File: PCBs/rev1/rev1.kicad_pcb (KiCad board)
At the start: 2 copper layers, 30.5 x 30.5 mm, 42 parts, among them J1 USB_B_Micro, J2 Conn_01x03, J3 Conn_01x08, J4 Conn_01x05, J5 Conn_01x04, J6 Conn_01x01, SW1 SW_Push, U1 RP2040, U2 AZ1117-3.3, U3 W25Q32JVSS, Y1 12Mhz

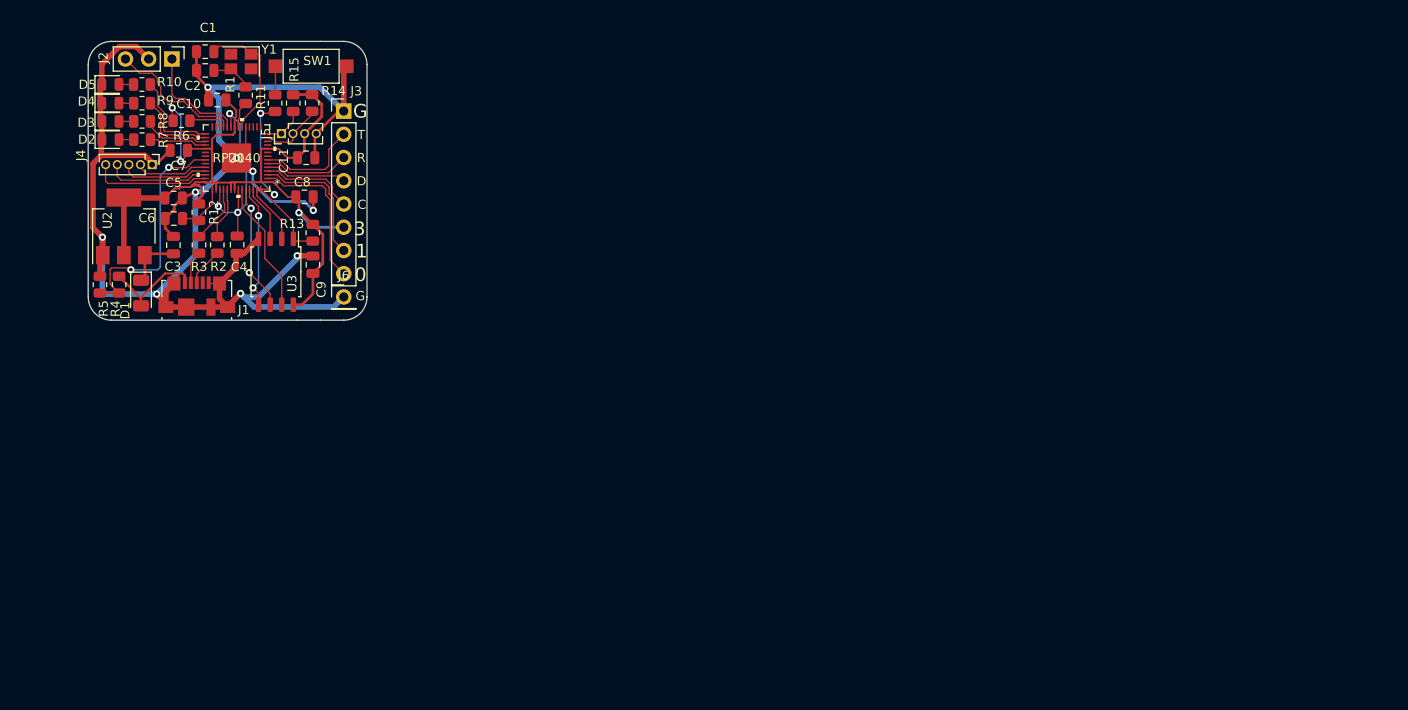
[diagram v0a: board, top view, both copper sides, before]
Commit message: PCB
dhwiqodhiowq
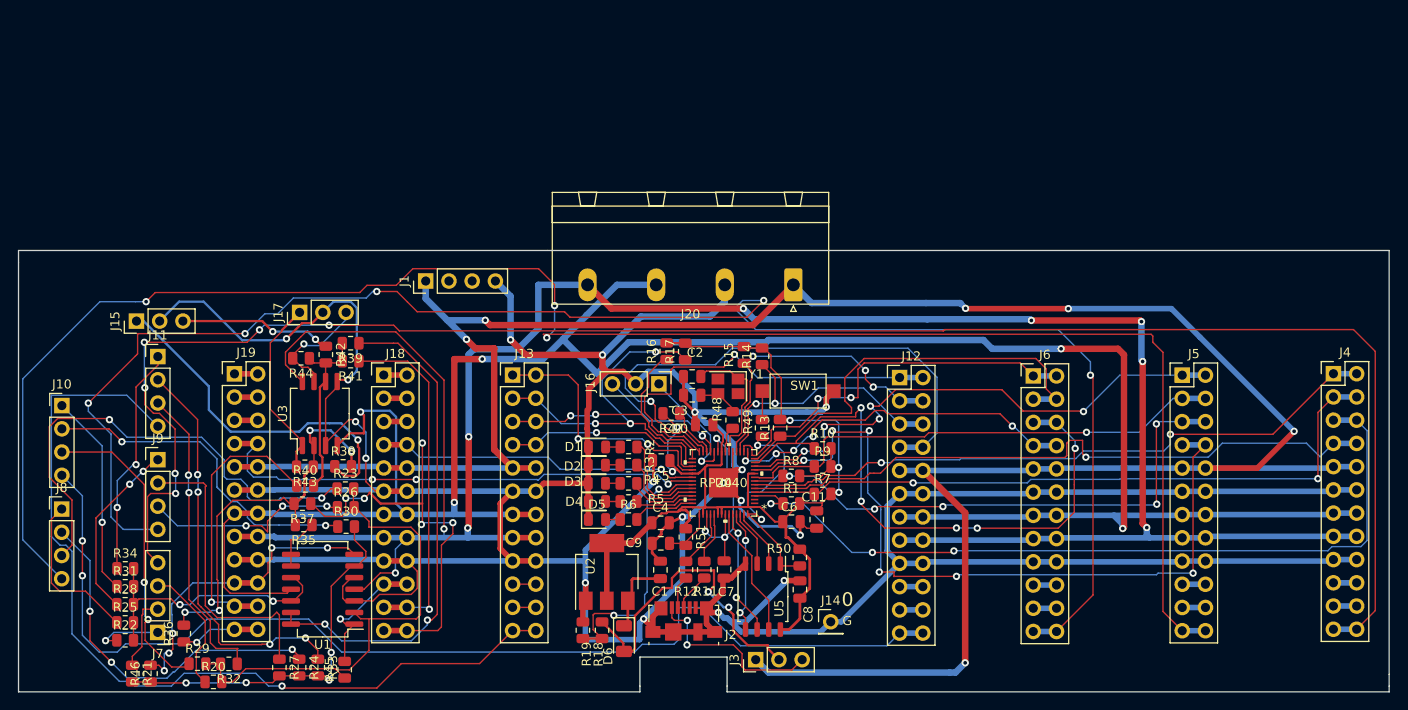
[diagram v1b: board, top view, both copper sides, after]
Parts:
- added D5: LED, LED_SMD:LED_0805_2012Metric, F.Cu at (182.6, 123.4)
- added J1: USB_A, Connector_PinHeader_2.54mm:PinHeader_1x04_P2.54mm_Vertical, F.Cu at (163.9, 97.3)
- added J10: Conn_01x04, Connector_PinHeader_2.54mm:PinHeader_1x04_P2.54mm_Vertical, F.Cu at (124.1, 110.9)
- added J11: Conn_01x04, Connector_PinHeader_2.54mm:PinHeader_1x04_P2.54mm_Vertical, F.Cu at (134.6, 105.6)
- added J12: Conn_02x12, Connector_PinHeader_2.54mm:PinHeader_2x12_P2.54mm_Vertical, F.Cu at (215.7, 107.9)
- added J13: Conn_02x12, Connector_PinHeader_2.54mm:PinHeader_2x12_P2.54mm_Vertical, F.Cu at (173.4, 107.6)
- added J15: Conn_01x03, Connector_PinHeader_2.54mm:PinHeader_1x03_P2.54mm_Vertical, F.Cu at (132.3, 101.7)
- added J17: Conn_01x03, Connector_PinHeader_2.54mm:PinHeader_1x03_P2.54mm_Vertical, F.Cu at (150.1, 100.8)
- added J18: Conn_02x12, Connector_PinHeader_2.54mm:PinHeader_2x12_P2.54mm_Vertical, F.Cu at (159.3, 107.6)
- added J19: Conn_02x12, Connector_PinHeader_2.54mm:PinHeader_2x12_P2.54mm_Vertical, F.Cu at (143.0, 107.5)
- added J20: Conn_01x04, Connector_Phoenix_GMSTB:PhoenixContact_GMSTBA_2,5_4-G_1x04_P7.50mm_Horizontal, F.Cu at (204.1, 97.7)
- added J6: Conn_02x12, Connector_PinHeader_2.54mm:PinHeader_2x12_P2.54mm_Vertical, F.Cu at (230.3, 107.7)
- added J7: Conn_01x04, Connector_PinHeader_2.54mm:PinHeader_1x04_P2.54mm_Vertical, F.Cu at (134.6, 135.7)
- added J8: Conn_01x04, Connector_PinHeader_2.54mm:PinHeader_1x04_P2.54mm_Vertical, F.Cu at (124.1, 122.2)
- added J9: Conn_01x04, Connector_PinHeader_2.54mm:PinHeader_1x04_P2.54mm_Vertical, F.Cu at (134.6, 116.9)
- added R1: R, Resistor_SMD:R_0805_2012Metric, F.Cu at (203.9, 121.7)
- added R10: R, Resistor_SMD:R_0805_2012Metric, F.Cu at (207.3, 115.6)
- added R13: R, Resistor_SMD:R_0805_2012Metric, F.Cu at (202.7, 113.4)
- added R16: R, Resistor_SMD:R_0805_2012Metric, F.Cu at (190.2, 105.0)
- added R17: R, Resistor_SMD:R_0805_2012Metric, F.Cu at (192.3, 105.0)
- added R20: R, Resistor_SMD:R_0805_2012Metric, F.Cu at (140.7, 141.2)
- added R21: R, Resistor_SMD:R_0805_2012Metric, F.Cu at (131.8, 140.2)
- added R22: R, Resistor_SMD:R_0805_2012Metric, F.Cu at (131.0, 136.6)
- added R23: R, Resistor_SMD:R_0805_2012Metric, F.Cu at (155.1, 120.0)
- added R24: R, Resistor_SMD:R_0805_2012Metric, F.Cu at (150.1, 139.6)
- added R25: R, Resistor_SMD:R_0805_2012Metric, F.Cu at (131.0, 134.7)
- added R26: R, Resistor_SMD:R_0805_2012Metric, F.Cu at (155.2, 122.1)
- added R27: R, Resistor_SMD:R_0805_2012Metric, F.Cu at (147.9, 139.6)
- added R28: R, Resistor_SMD:R_0805_2012Metric, F.Cu at (131.0, 132.7)
- added R29: R, Resistor_SMD:R_0805_2012Metric, F.Cu at (138.9, 139.2)
- added R30: R, Resistor_SMD:R_0805_2012Metric, F.Cu at (155.2, 124.2)
- added R31: R, Resistor_SMD:R_0805_2012Metric, F.Cu at (131.1, 130.7)
- added R32: R, Resistor_SMD:R_0805_2012Metric, F.Cu at (142.4, 139.2)
- added R33: R, Resistor_SMD:R_0805_2012Metric, F.Cu at (152.1, 139.6)
- added R34: R, Resistor_SMD:R_0805_2012Metric, F.Cu at (131.1, 128.7)
- added R35: R, Resistor_SMD:R_0805_2012Metric, F.Cu at (150.6, 124.0)
- added R36: R, Resistor_SMD:R_0805_2012Metric, F.Cu at (137.4, 135.9)
- added R37: R, Resistor_SMD:R_0805_2012Metric, F.Cu at (150.4, 121.7)
- added R38: R, Resistor_SMD:R_0805_2012Metric, F.Cu at (154.9, 117.6)
- added R39: R, Resistor_SMD:R_0805_2012Metric, F.Cu at (155.7, 104.1)
- added R40: R, Resistor_SMD:R_0805_2012Metric, F.Cu at (150.7, 119.7)
- added R41: R, Resistor_SMD:R_0805_2012Metric, F.Cu at (155.7, 106.1)
- added R42: R, Resistor_SMD:R_0805_2012Metric, F.Cu at (153.0, 105.4)
- added R43: R, Resistor_SMD:R_0805_2012Metric, F.Cu at (150.7, 117.6)
- added R44: R, Resistor_SMD:R_0805_2012Metric, F.Cu at (150.3, 105.8)
- added R45: R, Resistor_SMD:R_0805_2012Metric, F.Cu at (155.0, 139.8)
- added R46: R, Resistor_SMD:R_0805_2012Metric, F.Cu at (133.8, 140.2)
- added R6: 1K, Resistor_SMD:R_0805_2012Metric, F.Cu at (186.1, 123.4)
- added R7: R, Resistor_SMD:R_0805_2012Metric, F.Cu at (207.3, 120.6)
- added R8: R, Resistor_SMD:R_0805_2012Metric, F.Cu at (203.9, 118.6)
- added R9: R, Resistor_SMD:R_0805_2012Metric, F.Cu at (207.3, 117.6)
- added U1: TL074, Package_SO:SO-14_5.3x10.2mm_P1.27mm, F.Cu at (152.6, 131.0)
- added U3: TL072, Package_SO:SO-8_5.3x6.2mm_P1.27mm, F.Cu at (152.3, 111.8)
- J3: value Conn_01x08 -> Conn_01x03; footprint Connector_PinHeader_2.54mm:PinHeader_1x08_P2.54mm_Vertical -> Connector_PinHeader_2.54mm:PinHeader_1x03_P2.54mm_Vertical
- J4: value Conn_01x05 -> Conn_02x12_Odd_Even; footprint Connector_PinHeader_1.27mm:PinHeader_1x05_P1.27mm_Vertical -> Connector_PinHeader_2.54mm:PinHeader_2x12_P2.54mm_Vertical
- J5: value Conn_01x04 -> Conn_02x12; footprint Connector_PinHeader_1.27mm:PinHeader_1x04_P1.27mm_Vertical -> Connector_PinHeader_2.54mm:PinHeader_2x12_P2.54mm_Vertical
- R14, R15: value 4.7K -> R
- moved J4 131.2 mm to (263.1, 107.5), turned to 0 degrees
- moved J5 102.0 mm to (246.6, 107.6), turned to 0 degrees
- moved J3 75.0 mm to (200.0, 138.7), turned to 90 degrees
- moved D4 70.1 mm to (182.6, 121.4)
- moved R5 70.1 mm to (186.1, 121.4)
- moved C11 68.4 mm to (206.7, 123.4), turned to -90 degrees
- moved D3 67.5 mm to (182.6, 119.4)
- moved R4 67.5 mm to (186.1, 119.4)
- moved D2 65.1 mm to (182.6, 117.5)
- moved R3 65.1 mm to (186.1, 117.5)
- moved D6 64.9 mm to (185.6, 136.4)
- moved R18 64.9 mm to (183.2, 135.5)
- moved R19 64.9 mm to (181.1, 135.5)
- moved U2 64.9 mm to (183.7, 129.1)
- moved C7 64.0 mm to (196.5, 128.9)
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- renumbered C3 to C1, C1 to C2, C2 to C3, C5 to C4, C7 to C5, C8 to C6, C4 to C7, C9 to C8, C6 to C9, D2 to D1, D3 to D2, D4 to D3, D5 to D4, D1 to D6, J6 to J14, J2 to J16, J1 to J2, R2 to R11, R3 to R12, R4 to R18, R5 to R19, R7 to R2, R8 to R3, R9 to R4, R6 to R47, R1 to R48, R11 to R49, R10 to R5, R13 to R50, R12 to R51, U1 to U4, U3 to U5
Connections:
- net +5V renamed Net-(C1-Pad1)
- D6 pad 2: Net-(D1-Pad2) (its old number) -> Net-(D6-Pad2)
- J2 pad 1: Net-(D1-Pad2) (its old number) -> Net-(J2-Pad1)
- J2 pad 4: (no net) -> unconnected-(J2-Pad4)
- J3 pad 1: GND -> 5V
- J3 pad 2: GPIO5 -> Net-(D6-Pad2)
- J3 pad 3: GPIO4 -> Net-(J2-Pad1)
- J4 pad 1: GND -> GPIO5
- J4 pad 2: GPIO26 -> GPIO5
- J4 pad 3: GPIO27 -> GPIO3
- J4 pad 4: GPIO28 -> GPIO3
- J4 pad 5: GPIO29 -> GPIO2
- J5 pad 1: GPIO11 -> GPIO9
- J5 pad 2: GPIO10 -> GPIO9
- J5 pad 3: +3V3 -> GPIO7
- J5 pad 4: GND -> GPIO7
- R14 pad 1: GPIO10 -> GPIO14
- R15 pad 1: GPIO11 -> GPIO15
- R18 pad 1: Net-(D1-Pad2) (its old number) -> Net-(D6-Pad2)
- R2 pad 2: GPIO21 -> GPIO25
- R3 pad 2: GPIO20 -> GPIO26
- R4 pad 2: GPIO19 -> GPIO27
- R5 pad 2: GPIO18 -> GPIO28
- U4 pad 11: (no net) -> DET_2
- U4 pad 12: (no net) -> GPIO9
- U4 pad 15: (no net) -> DET_3
- U4 pad 16: (no net) -> GPIO13
- U4 pad 17: (no net) -> GPIO14
- U4 pad 18: (no net) -> GPIO15
- U4 pad 27: (no net) -> DET_4
- U4 pad 28: (no net) -> GPIO17
- U4 pad 31: GPIO20 -> DET_5
- U4 pad 34: (no net) -> DET_A
- U4 pad 35: (no net) -> DET_B
- U4 pad 37: (no net) -> GPIO25
- U4 pad 6: GPIO4 -> DET_1
- U4 pad 8: (no net) -> GPIO6
- U4 pad 9: (no net) -> GPIO7
- Y1 pad 2: (no net) -> unconnected-(Y1-Pad2)
- Y1 pad 4: (no net) -> unconnected-(Y1-Pad4)
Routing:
- net GND: track 188.6 -> 509.3 mm, vias 9 -> 18
- net 5V: track 0.00 -> 268.3 mm, vias 0 -> 6
- net +12V: track 0.00 -> 259.8 mm, vias 0 -> 9
- net -12V: track 0.00 -> 249.6 mm, vias 0 -> 5
- net A_OUT_L_1: track 0.00 -> 199.8 mm, vias 0 -> 6
- net A_OUT_L_2: track 0.00 -> 197.0 mm, vias 0 -> 3
- net A_OUT_L_3: track 0.00 -> 179.7 mm, vias 0 -> 5
- net A_OUT_L_4: track 0.00 -> 120.4 mm, vias 0 -> 2
- net A_OUT_L_5: track 0.00 -> 97.3 mm, vias 0 -> 1
- net DET_2: track 0.00 -> 84.4 mm, vias 0 -> 6
- net GPIO2: track 10.3 -> 88.9 mm, vias 0 -> 3
- net DET_1: track 0.00 -> 72.3 mm, vias 0 -> 1
- net GPIO3: track 8.93 -> 74.6 mm, vias 0 -> 2
- net DET_4: track 0.00 -> 61.5 mm, vias 0 -> 1
- net GPIO5: track 11.4 -> 71.7 mm, vias 0 -> 2
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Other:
- board size 30.5 x 30.5 mm -> 149.9 x 48.3 mm
- net class Default removed
- board text added: "A_OUT_L_1"
- board text added: "A_OUT_L_2"
- board text added: "A_OUT_L_3"
- board text added: "A_OUT_L_4"
- board text added: "A_OUT_L_5"
- board text added: "DAC"
- board text added: "DRUM 1"
- board text added: "DRUM 2"
- board text added: "DRUM 3"
- board text added: "DRUM 4"
- board text added: "DRUM 5"
- board text added: "EFFECT A"
- board text added: "EFFECT B"
- board text added: "FILTER"
- board text added: "USB-A"
- board text removed: "1"
- board text removed: "3"
- board text removed: "3V3"
- board text removed: "5"
- board text removed: "C"
- board text removed: "D"
- board text removed: "GND"
- board text removed: "GPIO0"
- board text removed: "GPIO1"
- board text removed: "GPIO10"
- board text removed: "GPIO11"
- board text removed: "GPIO2"
- board text removed: "GPIO26"
- board text removed: "GPIO27"
- board text removed: "GPIO28"
- board text removed: "GPIO29"
- board text removed: "GPIO3"
- board text removed: "GPIO4"
- board text removed: "R"
- board text removed: "RP2040 10/16/21 MARK"
- board text removed: "SWCLK"
- board text removed: "SWDIO"
- board text removed: "T"
